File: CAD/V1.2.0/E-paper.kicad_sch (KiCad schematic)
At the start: 44 parts, among them K12 SFV6R-1STBE1HLF, K13 SFV34R-3STBE1HLF, K36 SFV8R-1STBE1HLF, Q10 PMOS, Q11 NMOS, Q12 PMOS, Q13 PMOS, U10 SN74LVC1G34DBV, U14 TXS0104EPWR, U15 ED060XH7, U8 MCP47A1, U9 AP5726WG-7

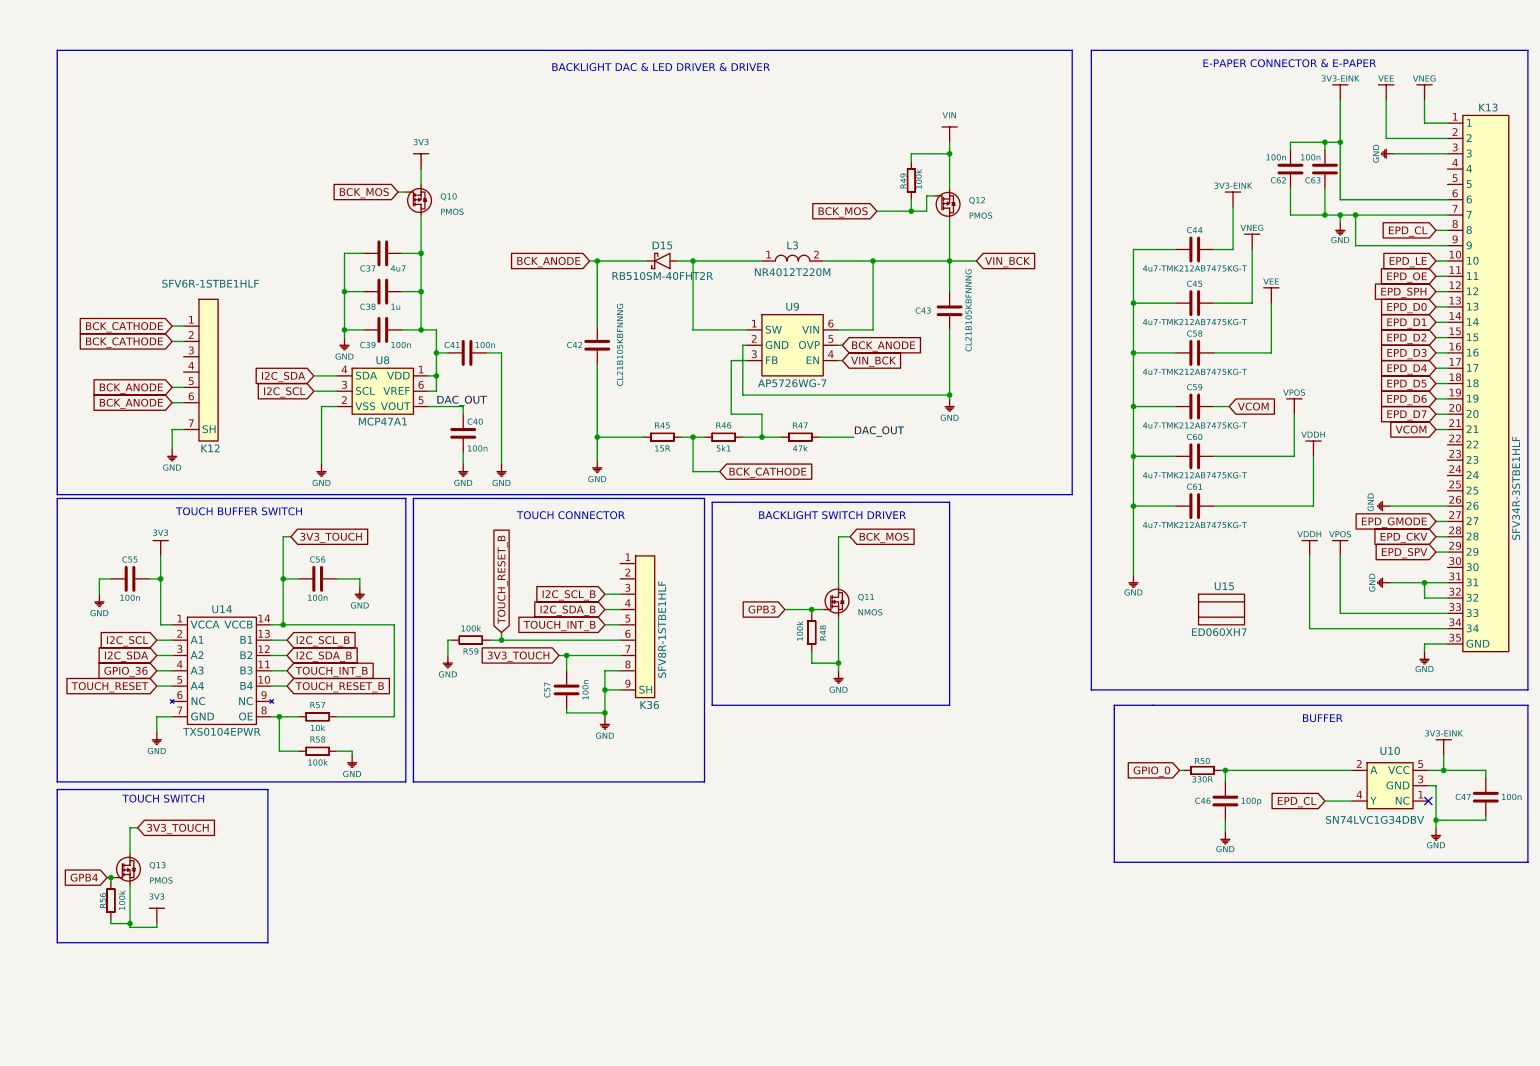
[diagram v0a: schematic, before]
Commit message: Updating open source files.
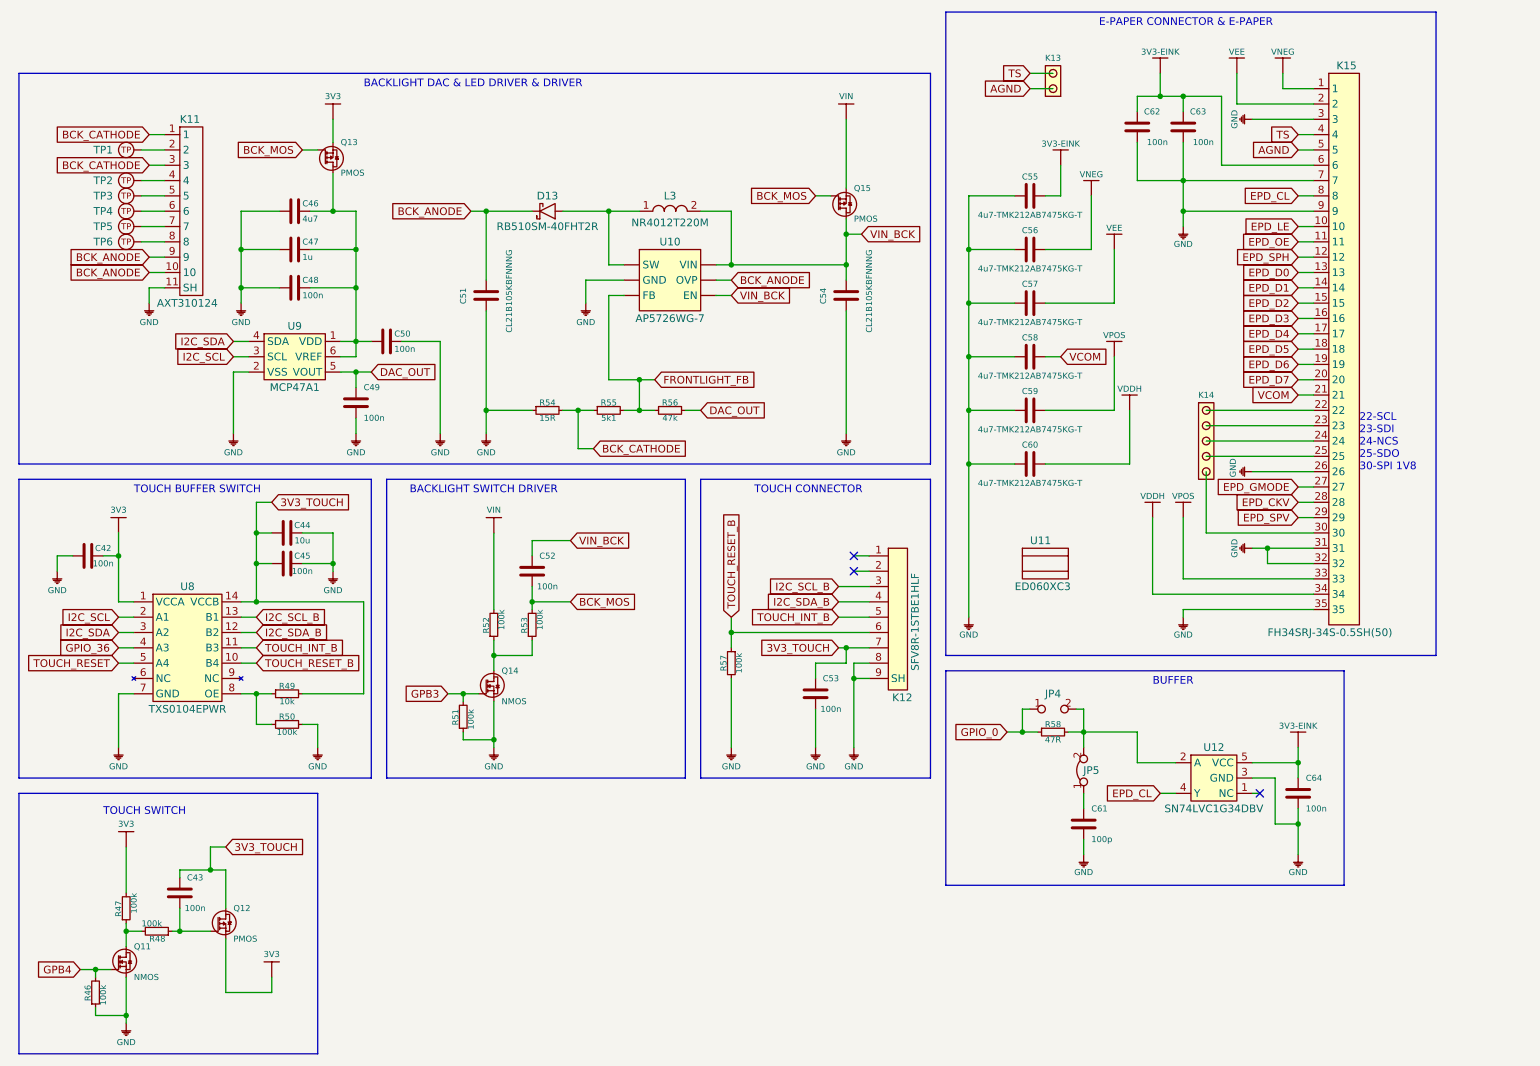
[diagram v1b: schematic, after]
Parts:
- removed K12: SFV6R-1STBE1HLF, e-radionica.com footprinti:SFV6R-1STBE1HLF, symbol e-radionica.com schematics:SFV6R-1STBE1HLF
- removed K13: SFV34R-3STBE1HLF, e-radionica.com footprinti:SFV34R-3STBE1HLF, symbol e-radionica.com schematics:SFV34R-3STBE1HLF
- removed R49, R56: 100k, e-radionica.com footprinti:0603R, symbol e-radionica.com schematics:0603R
- removed U15: ED060XH7, e-radionica.com footprinti:ED060XH7, symbol e-radionica.com schematics:ED060XH7
- added C43, C52: 100n, e-radionica.com footprinti:0603C, symbol e-radionica.com schematics:0603C
- added C44: 10u, e-radionica.com footprinti:1206C, symbol e-radionica.com schematics:1206C
- added JP4: SMD_JUMPER, e-radionica.com footprinti:SMD_JUMPER, symbol e-radionica.com schematics:SMD_JUMPER
- added JP5: SMD-JUMPER-CONNECTED_TRACE_SOLDERMASK, e-radionica.com footprinti:SMD-JUMPER-CONNECTED_TRACE_SOLDERMASK, symbol e-radionica.com schematics:SMD-JUMPER-CONNECTED_TRACE_SOLDERMASK
- added K11: AXT310124, e-radionica.com footprinti:AXT310124, symbol e-radionica.com schematics:AXT310124
- added K13: HEADER_MALE_2X1, e-radionica.com footprinti:HEADER_MALE_2X1, symbol e-radionica.com schematics:HEADER_MALE_2X1
- added K14: HEADER_MALE_5X1, e-radionica.com footprinti:HEADER_MALE_5X1, symbol e-radionica.com schematics:HEADER_MALE_5X1
- added K15: FH34SRJ-34S-0.5SH(50), e-radionica.com footprinti:FH34SRJ-34S-0.5SH(50), symbol e-radionica.com schematics:FH34SRJ-34S-0.5SH(50)
- added Q11: NMOS, e-radionica.com footprinti:SOT-23-3, symbol e-radionica.com schematics:NMOS-SOT-23-3
- added R46, R47, R48, R52, R53: 100k, e-radionica.com footprinti:0603R, symbol e-radionica.com schematics:0603R
- added TP1, TP2, TP3, TP4, TP5, TP6: Test_Point_SMD_0.8mm, e-radionica.com footprinti:Test_Point_SMD_0.8mm, symbol e-radionica.com schematics:Test_Point_SMD_0.8mm
- added U11: ED060XC3, e-radionica.com footprinti:ED060XC3, symbol e-radionica.com schematics:ED060XC3
- R58: renamed from R50; value 330R -> 47R
- renumbered C55 to C42, C56 to C45, C37 to C46, C38 to C47, C39 to C48, C40 to C49, C41 to C50, C42 to C51, C57 to C53, C43 to C54, C44 to C55, C45 to C56, C58 to C57, C59 to C58, C60 to C59, C61 to C60, C46 to C61, C47 to C64, D15 to D13, K36 to K12, Q13 to Q12, Q10 to Q13, Q11 to Q14, Q12 to Q15, R57 to R49, R58 to R50, R48 to R51, R45 to R54, R46 to R55, R47 to R56, R59 to R57, U9 to U10, U10 to U12, U14 to U8, U8 to U9
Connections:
- net 3V3: now also R47.2
- net 3V3-EINK: now also K15.6
- net 3V3_TOUCH: now also C43.2, C44.1
- net BCK_ANODE: now also K11.10, K11.9
- net BCK_CATHODE: now also K11.1, K11.3
- net BCK_MOS: now also C52.1, R53.2; no longer Q14.3 (D)
- net EPD_CKV: now also K15.28
- net EPD_CL: now also K15.8
- net EPD_D0: now also K15.13
- net EPD_D1: now also K15.14
- net EPD_D2: now also K15.15
- net EPD_D3: now also K15.16
- net EPD_D4: now also K15.17
- net EPD_D5: now also K15.18
- net EPD_D6: now also K15.19
- net EPD_D7: now also K15.20
- net EPD_GMODE: now also K15.27
- net EPD_LE: now also K15.10
- net EPD_OE: now also K15.11
- net EPD_SPH: now also K15.12
- net EPD_SPV: now also K15.29
- net GND: now also C44.2, K11.11 (SH), K15.26, K15.3, K15.31, K15.32, K15.35, K15.7, K15.9, Q11.2 (S), R46.1
- net GPB4: now also Q11.1 (G), R46.2; no longer Q12.1 (G)
- net GPIO_0: now also JP4.1
- net VCOM: now also K15.21
- net VDDH: now also K15.34
- net VEE: now also K15.2
- net VIN: now also R52.2
- net VIN_BCK: now also C52.2
- net VNEG: now also K15.1
- net VPOS: now also K15.33
- net FRONTLIGHT_FB: now reaches R55.2, R56.1, U10.3 (FB)
- net at R58.2, U12.2 (A): now also JP4.2, JP5.2; no longer C61.2
- new net: K11.8, TP6.TP
- new net: C43.1, Q12.1 (G), R48.1
- new net: K14.1, K15.30
- new net: K14.2, K15.25
- new net: K14.3, K15.24
- new net: K14.4, K15.23
- new net: K14.5, K15.22
- new net: K11.2, TP1.TP
- new net: K11.4, TP2.TP
- new net: Q14.3 (D), R52.1, R53.1
- new net: Q11.3 (D), R47.1, R48.2
- new net: K11.7, TP5.TP
- new net: K11.6, TP4.TP
- new net: C61.2, JP5.1
- new net: K11.5, TP3.TP
- new net AGND: K13.1, K15.5
- new net TS: K13.2, K15.4
- no-connect marks 1 -> 3
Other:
- note added: "22-SCL 23-SDI 24-NCS 25-SDO 30-SPI 1V8"
- title: Soldered Inkplate 6PLUS -> Soldered Inkplate 6 FLICK
- moved on the sheet: C42, C45, C46, C47, C48, C49, C50, C51, C53, C54, C55, C56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
